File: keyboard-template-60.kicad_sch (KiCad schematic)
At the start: 180 parts, among them J1 USB_C_Receptacle_USB2.0, J2 Conn_01x04_MountingPin, J3 AVR-ISP-6, J4 Conn_01x08_Pin, SW1 SW_Reset, U1 ATmega32U4-M, U2 SRV05-4, U3 TP_Sprintek_SK8707-01_Sensor, U5 TXS0102DCU, U6 AMS1117-3.3, Y1 16MHz

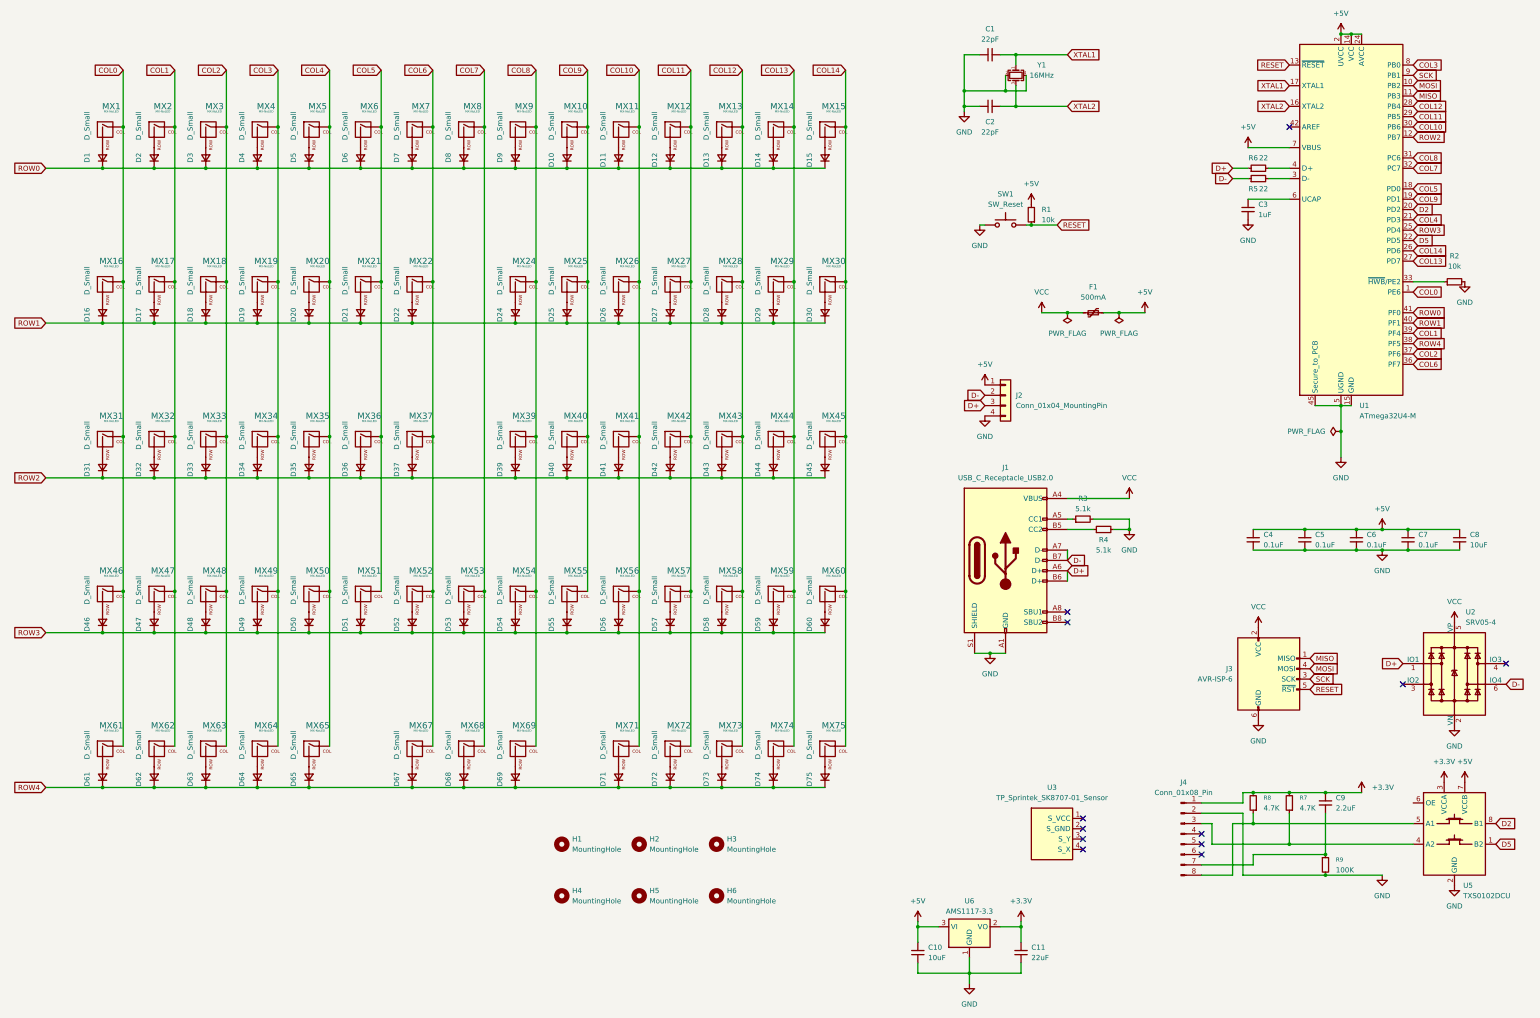
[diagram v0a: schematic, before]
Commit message: Tracing of the new schematic layout
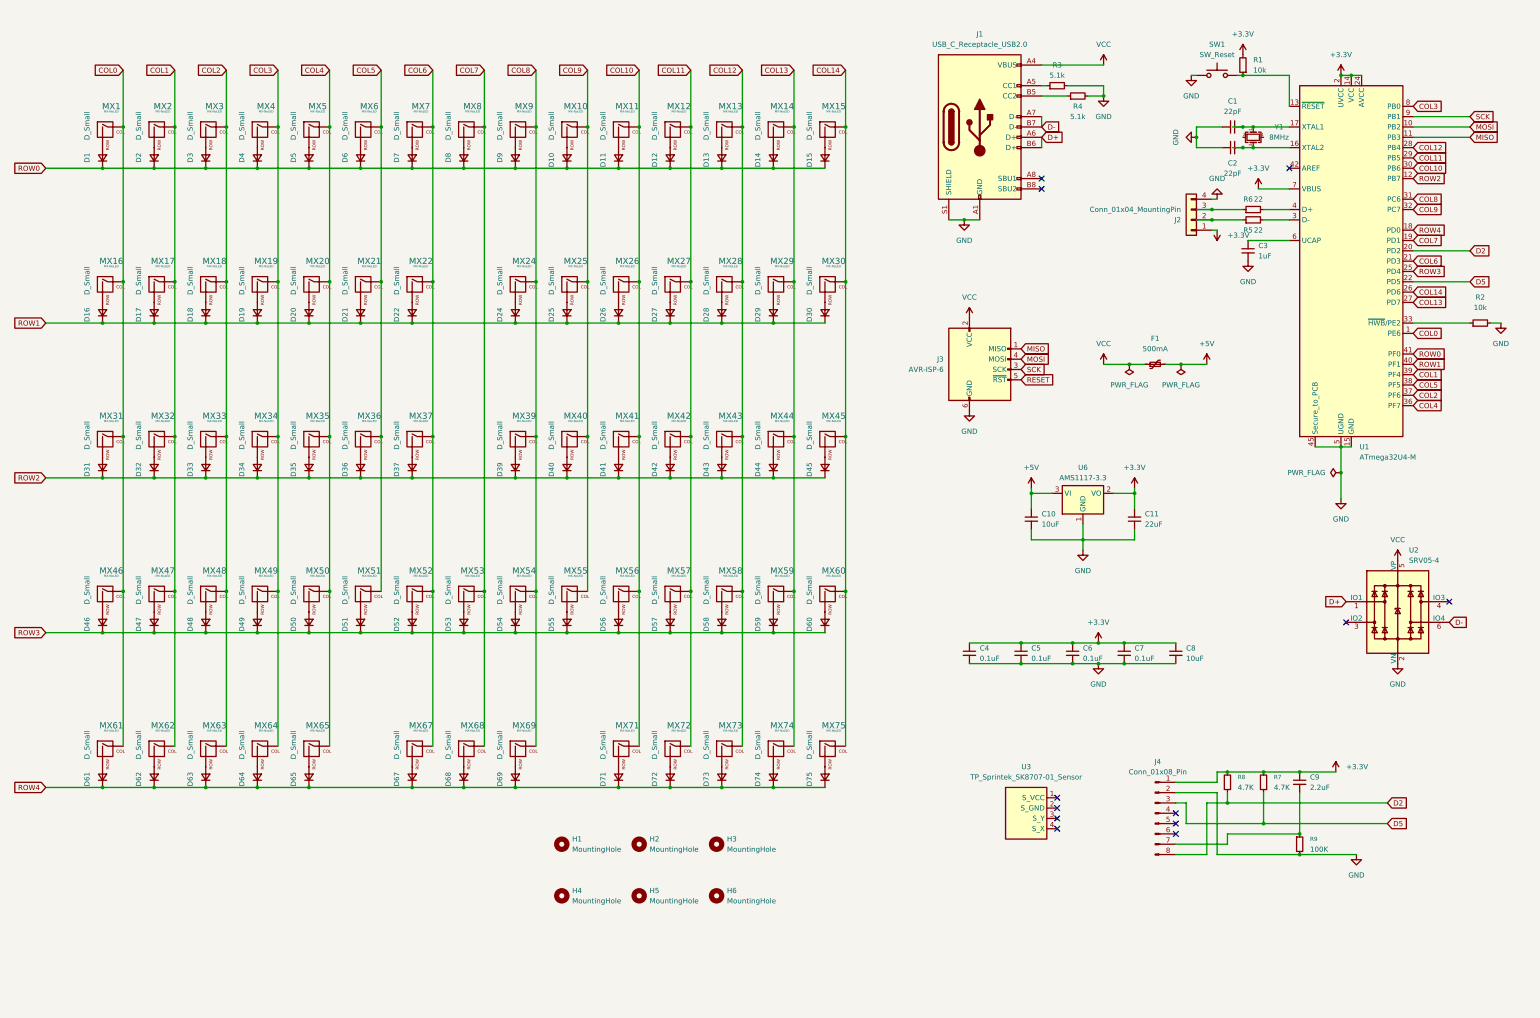
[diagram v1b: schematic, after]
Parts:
- removed U5: TXS0102DCU, Package_SO:VSSOP-8_2.3x2mm_P0.5mm, symbol Logic_LevelTranslator:TXS0102DCU
- MX1, MX10, MX11, MX12, MX13, MX14, MX15, MX16, MX17, MX18, MX19, MX2, MX20, MX21, MX22, MX24, MX25, MX26, MX27, MX28, MX29, MX3, MX30, MX31, MX32, MX33, MX34, MX35, MX36, MX37, MX39, MX4, MX40, MX41, MX42, MX43, MX44, MX45, MX46, MX47, MX48, MX49, MX5, MX50, MX51, MX52, MX53, MX54, MX55, MX56, MX57, MX58, MX59, MX6, MX60, MX61, MX62, MX63, MX64, MX65, MX7, MX71, MX72, MX73, MX74, MX75, MX8, MX9: footprint MX_Only:MXOnly-1U-Hotswap-Antishear -> MX_Only:MXOnly-1U-Hotswap
- Y1: value 16MHz -> 8MHz
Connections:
- net +3.3V: now also C4.1, C5.1, C6.1, C7.1, C8.1, J2.1 (Pin_1), R1.2, U1.14 (VCC), U1.2 (UVCC), U1.24 (AVCC), U1.34 (VCC), U1.44 (AVCC), U1.7 (VBUS)
- net +5V: no longer C4.1, C5.1, C6.1, C7.1, C8.1, J2.1 (Pin_1), R1.2, U1.14 (VCC), U1.2 (UVCC), U1.24 (AVCC), U1.34 (VCC), U1.44 (AVCC), U1.7 (VBUS)
- net COL4: now also U1.36 (PF7); no longer U1.21 (PD3)
- net COL5: now also U1.38 (PF5); no longer U1.18 (PD0)
- net COL6: now also U1.21 (PD3); no longer U1.36 (PF7)
- net COL7: now also U1.19 (PD1); no longer U1.32 (PC7)
- net COL9: now also U1.32 (PC7); no longer U1.19 (PD1)
- net D+: no longer J2.3 (Pin_3), R6.1
- net D-: no longer J2.2 (Pin_2), R5.1
- net D2: now also J4.8 (Pin_8), R8.1
- net D5: now also J4.3 (Pin_3), R7.1
- net GND: no longer Y1.2, Y1.4
- net RESET: no longer R1.1, SW1.2, U1.13 (~{RESET})
- net ROW4: now also U1.18 (PD0); no longer U1.38 (PF5)
- net XTAL1: no longer names the net of C1.2, U1.17 (XTAL1), Y1.1
- net XTAL2: no longer names the net of C2.2, U1.16 (XTAL2), Y1.3
- new net: J2.2 (Pin_2), R5.1
- new net: J2.3 (Pin_3), R6.1
- new net: R1.1, SW1.2, U1.13 (~{RESET})
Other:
- moved on the sheet: C1, C10, C11, C2, C3, C4, C5, C6, C7, C8, C9, F1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

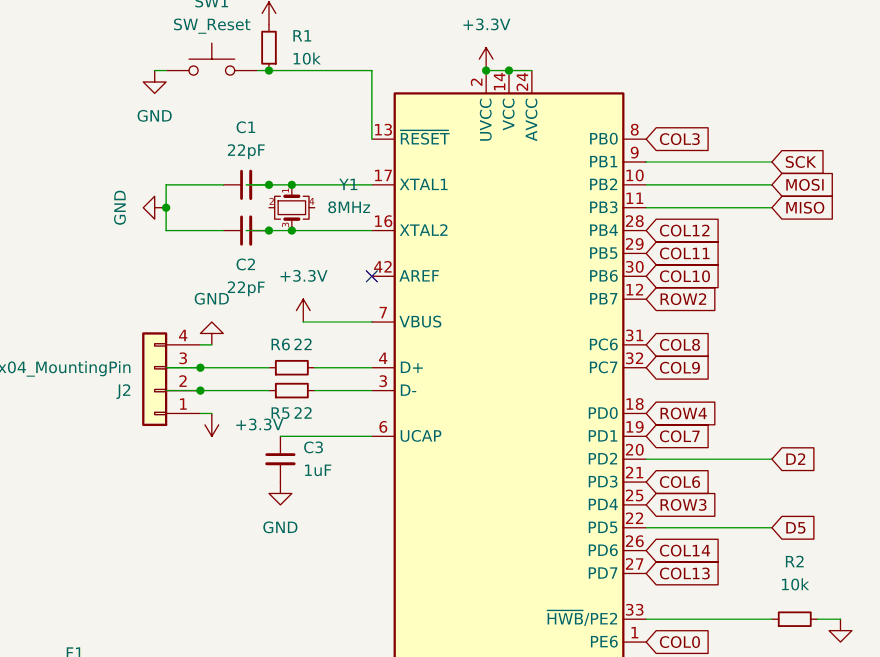
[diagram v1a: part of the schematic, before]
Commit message: More retracing
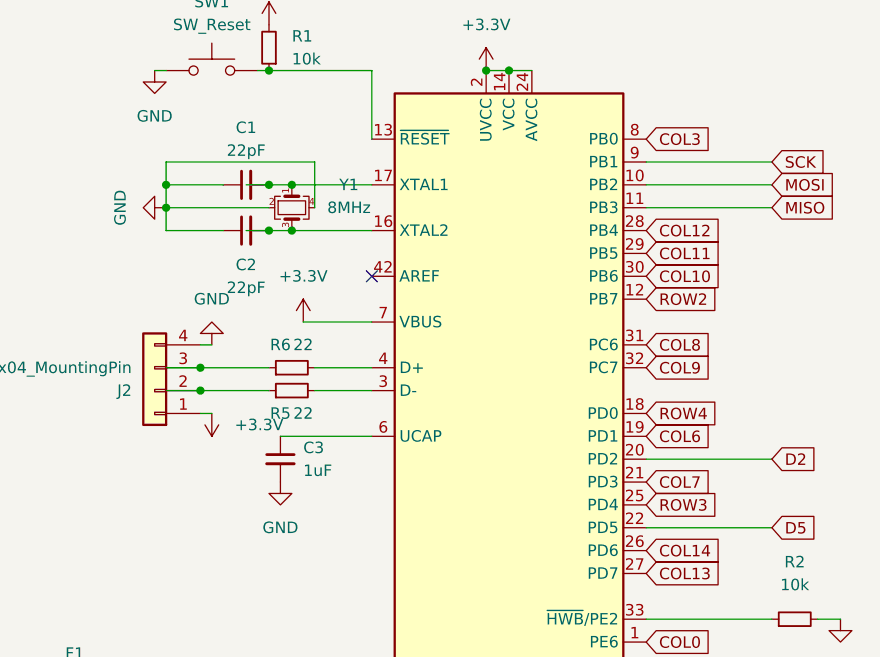
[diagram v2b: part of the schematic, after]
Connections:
- net COL6: now also U1.19 (PD1); no longer U1.21 (PD3)
- net COL7: now also U1.21 (PD3); no longer U1.19 (PD1)
- net GND: now also Y1.2, Y1.4
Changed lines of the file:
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@@
 	)
 	(junction
+		(at 321.31 52.07)
+		(diameter 0)
+		(color 0 0 0 0)
+	)
+	(junction
 		(at 179.07 62.23)
 		(diameter 0)
@@
 	(wire
 		(pts
+			(xy 321.31 54.61) (xy 332.74 54.61)
+		)
+		(stroke
+			(width 0)
+			(type default)
+		)
+	)
+	(wire
+		(pts
 			(xy 278.13 184.15) (xy 290.83 184.15)
 		)
@@
 	(wire
 		(pts
+			(xy 337.82 49.53) (xy 321.31 49.53)
+		)
+		(stroke
+			(width 0)
+			(type default)
+		)
+	)
+	(wire
+		(pts
 			(xy 52.07 100.33) (xy 64.77 100.33)
 		)
@@
 	(wire
 		(pts
+			(xy 321.31 49.53) (xy 321.31 52.07)
+		)
+		(stroke
+			(width 0)
+			(type default)
+		)
+	)
+	(wire
+		(pts
 			(xy 326.39 210.82) (xy 328.93 210.82)
 		)
@@
 	(wire
 		(pts
+			(xy 337.82 54.61) (xy 337.82 49.53)
+		)
+		(stroke
+			(width 0)
+			(type default)
+		)
+	)
+	(wire
+		(pts
 			(xy 107.95 166.37) (xy 107.95 204.47)
 		)
@@
 	(global_label "COL6"
 		(shape input)
-		(at 374.65 85.09 0)
+		(at 374.65 80.01 0)
 		(fields_autoplaced yes)
 		(effects
@@
 		)
 		(property "Intersheetrefs" "${INTERSHEET_REFS}"
-			(at 381.9012 85.1694 0)
+			(at 381.9012 80.0894 0)
 			(effects
 				(font
@@
 	(global_label "COL7"
 		(shape input)
-		(at 374.65 80.01 0)
+		(at 374.65 85.09 0)
 		(fields_autoplaced yes)
 		(effects
@@
 		)
 		(property "Intersheetrefs" "${INTERSHEET_REFS}"
-			(at 381.9012 80.0894 0)
+			(at 381.9012 85.1694 0)
 			(effects
 				(font
